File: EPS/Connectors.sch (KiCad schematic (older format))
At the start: 1 part

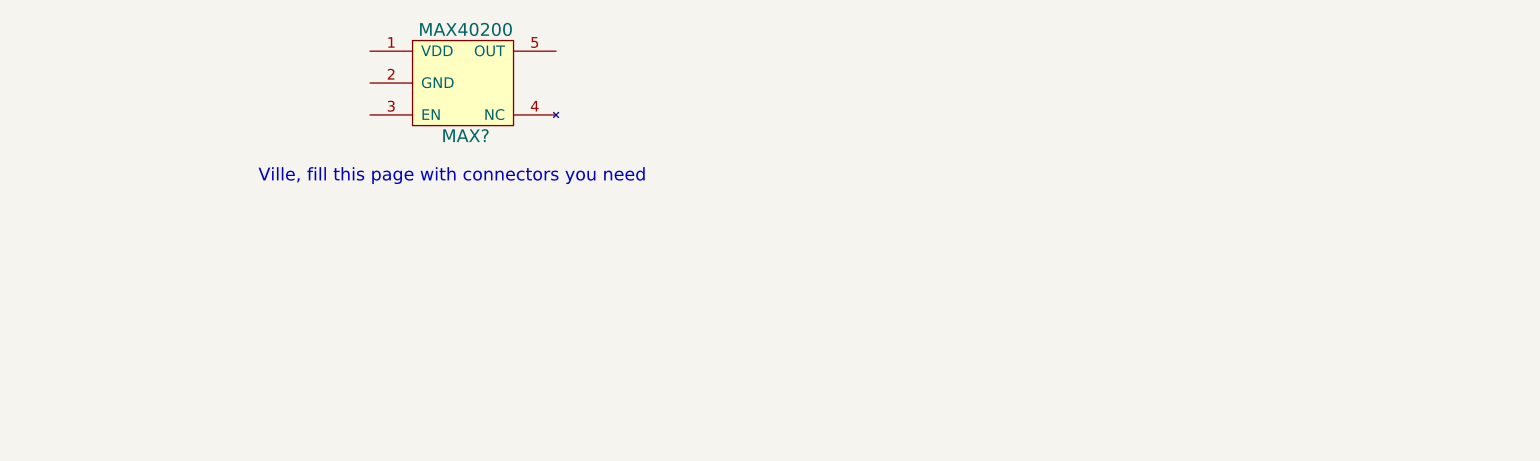
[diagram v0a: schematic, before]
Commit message: Updated schematics
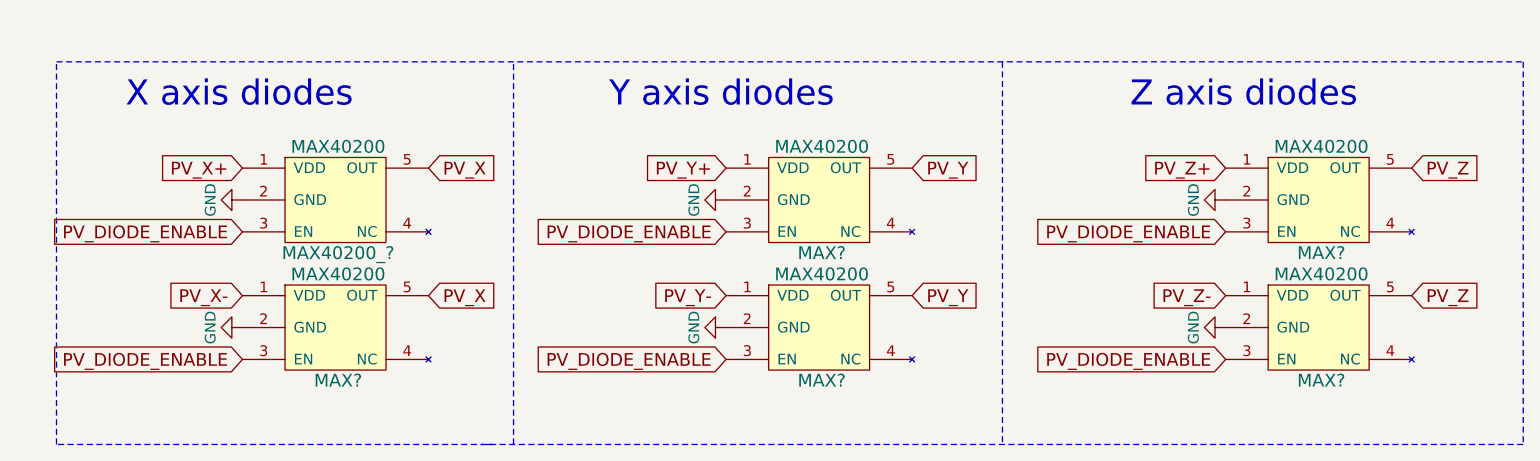
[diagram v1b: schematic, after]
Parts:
- added MAX40200_?, MAX? (x4): MAX40200, symbol MAX40200
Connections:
- net PV_X-: now reaches MAX?.1 (VDD)
- net GND: now reaches MAX?.2 (GND)
- net GND: now also MAX40200_?.2 (GND), MAX?.2 (GND), MAX?.2 (GND), MAX?.2 (GND), MAX?.2 (GND)
- net PV_DIODE_ENABLE: now reaches MAX?.3 (EN)
- net PV_DIODE_ENABLE: now also MAX40200_?.3 (EN), MAX?.3 (EN), MAX?.3 (EN), MAX?.3 (EN), MAX?.3 (EN)
- net PV_X: now reaches MAX?.5 (OUT)
- net PV_X: now also MAX40200_?.5 (OUT)
- new net PV_X+: MAX40200_?.1 (VDD)
- new net PV_Y: MAX?.5 (OUT), MAX?.5 (OUT)
- new net PV_Y+: MAX?.1 (VDD)
- new net PV_Y-: MAX?.1 (VDD)
- new net PV_Z: MAX?.5 (OUT), MAX?.5 (OUT)
- new net PV_Z+: MAX?.1 (VDD)
- new net PV_Z-: MAX?.1 (VDD)
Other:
- note added: "X axis diodes"
- note added: "Y axis diodes"
- note added: "Z axis diodes"
- note removed: "Ville, fill this page with connectors you need\n"
- moved on the sheet: MAX?
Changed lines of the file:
@@
 LIBS:max40200
 LIBS:tps7a7002
+LIBS:max5395
 LIBS:EPS-cache
 EELAYER 25 0
@@
 L MAX40200 MAX?
 U 1 1 5A8C9975
-P 5525 2725
-F 0 "MAX?" H 5525 2450 60  0000 C CNN
-F 1 "MAX40200" H 5525 2950 60  0000 C CNN
-F 2 "" H 5475 2725 60  0001 C CNN
-F 3 "" H 5475 2725 60  0001 C CNN
-	1    5525 2725
-	1    0    0    -1
-$EndComp
-Text Notes 4550 3225 0    60   ~ 0
-Ville, fill this page with connectors you need\n
+P 4925 3875
+F 0 "MAX?" H 4925 3600 60  0000 C CNN
+F 1 "MAX40200" H 4925 4100 60  0000 C CNN
+F 2 "" H 4875 3875 60  0001 C CNN
+F 3 "" H 4875 3875 60  0001 C CNN
+	1    4925 3875
+	1    0    0    -1
+$EndComp
+$Comp
+L MAX40200 MAX40200_?
+U 1 1 5A8B6733
+P 4925 3275
+F 0 "MAX40200_?" H 4925 3000 60  0000 C CNN
+F 1 "MAX40200" H 4925 3500 60  0000 C CNN
+F 2 "" H 4875 3275 60  0001 C CNN
+F 3 "" H 4875 3275 60  0001 C CNN
+	1    4925 3275
+	1    0    0    -1
+$EndComp
+Wire Notes Line
+	3600 2650 10500 2650
+Wire Notes Line
+	10500 2650 10500 4450
+Wire Notes Line
+	10500 4450 3600 4450
+Wire Notes Line
+	3600 4450 3600 2650
+Wire Notes Line
+	5650 4450 5600 4450
+Wire Notes Line
+	8050 2650 8050 4450
+$Comp
+L MAX40200 MAX?
+U 1 1 5A8B6858
+P 7200 3875
+F 0 "MAX?" H 7200 3600 60  0000 C CNN
+F 1 "MAX40200" H 7200 4100 60  0000 C CNN
+F 2 "" H 7150 3875 60  0001 C CNN
+F 3 "" H 7150 3875 60  0001 C CNN
+	1    7200 3875
+	1    0    0    -1
+$EndComp
+$Comp
+L MAX40200 MAX?
+U 1 1 5A8B685E
+P 7200 3275
+F 0 "MAX?" H 7200 3000 60  0000 C CNN
+F 1 "MAX40200" H 7200 3500 60  0000 C CNN
+F 2 "" H 7150 3275 60  0001 C CNN
+F 3 "" H 7150 3275 60  0001 C CNN
+	1    7200 3275
+	1    0    0    -1
+$EndComp
+$Comp
+L MAX40200 MAX?
+U 1 1 5A8B6906
+P 9550 3875
+F 0 "MAX?" H 9550 3600 60  0000 C CNN
+F 1 "MAX40200" H 9550 4100 60  0000 C CNN
+F 2 "" H 9500 3875 60  0001 C CNN
+F 3 "" H 9500 3875 60  0001 C CNN
+	1    9550 3875
+	1    0    0    -1
+$EndComp
+$Comp
+L MAX40200 MAX?
+U 1 1 5A8B690C
+P 9550 3275
+F 0 "MAX?" H 9550 3000 60  0000 C CNN
+F 1 "MAX40200" H 9550 3500 60  0000 C CNN
+F 2 "" H 9500 3275 60  0001 C CNN
+F 3 "" H 9500 3275 60  0001 C CNN
+	1    9550 3275
+	1    0    0    -1
+$EndComp
+Text GLabel 4475 3150 0    60   Input ~ 0
+PV_X+
+Text GLabel 4475 3750 0    60   Input ~ 0
+PV_X-
+Text GLabel 6750 3150 0    60   Input ~ 0
+PV_Y+
+Text GLabel 6750 3750 0    60   Input ~ 0
+PV_Y-
+Text GLabel 9100 3150 0    60   Input ~ 0
+PV_Z+
+Text GLabel 9100 3750 0    60   Input ~ 0
+PV_Z-
+Text GLabel 5350 3150 2    60   Input ~ 0
+PV_X
+Text GLabel 5350 3750 2    60   Input ~ 0
+PV_X
+Text GLabel 7625 3150 2    60   Input ~ 0
+PV_Y
+Text GLabel 7625 3750 2    60   Input ~ 0
+PV_Y
+Text GLabel 9975 3150 2    60   Input ~ 0
+PV_Z
+Text GLabel 9975 3750 2    60   Input ~ 0
+PV_Z
+$Comp
+L GND #PWR?
+U 1 1 5A8B7527
+P 4475 3300
+F 0 "#PWR?" H 4475 3050 50  0001 C CNN
+F 1 "GND" H 4475 3150 50  0000 C CNN
+F 2 "" H 4475 3300 50  0001 C CNN
+F 3 "" H 4475 3300 50  0001 C CNN
+	1    4475 3300
+	0    1    1    0
+$EndComp
+$Comp
+L GND #PWR?
+U 1 1 5A8B755E
+P 4475 3900
+F 0 "#PWR?" H 4475 3650 50  0001 C CNN
+F 1 "GND" H 4475 3750 50  0000 C CNN
+F 2 "" H 4475 3900 50  0001 C CNN
+F 3 "" H 4475 3900 50  0001 C CNN
+	1    4475 3900
+	0    1    1    0
+$EndComp
+$Comp
+L GND #PWR?
+U 1 1 5A8B757B
+P 6750 3300
+F 0 "#PWR?" H 6750 3050 50  0001 C CNN
+F 1 "GND" H 6750 3150 50  0000 C CNN
+F 2 "" H 6750 3300 50  0001 C CNN
+F 3 "" H 6750 3300 50  0001 C CNN
+	1    6750 3300
+	0    1    1    0
+$EndComp
+$Comp
+L GND #PWR?
+U 1 1 5A8B7598
+P 6750 3900
+F 0 "#PWR?" H 6750 3650 50  0001 C CNN
+F 1 "GND" H 6750 3750 50  0000 C CNN
+F 2 "" H 6750 3900 50  0001 C CNN
+F 3 "" H 6750 3900 50  0001 C CNN
+	1    6750 3900
+	0    1    1    0
+$EndComp
+$Comp
+L GND #PWR?
+U 1 1 5A8B75B5
+P 9100 3300
+F 0 "#PWR?" H 9100 3050 50  0001 C CNN
+F 1 "GND" H 9100 3150 50  0000 C CNN
+F 2 "" H 9100 3300 50  0001 C CNN
+F 3 "" H 9100 3300 50  0001 C CNN
+	1    9100 3300
+	0    1    1    0
+$EndComp
+$Comp
+L GND #PWR?
+U 1 1 5A8B75D2
+P 9100 3900
+F 0 "#PWR?" H 9100 3650 50  0001 C CNN
+F 1 "GND" H 9100 3750 50  0000 C CNN
+F 2 "" H 9100 3900 50  0001 C CNN
+F 3 "" H 9100 3900 50  0001 C CNN
+	1    9100 3900
+	0    1    1    0
+$EndComp
+Text GLabel 4475 3450 0    60   Input ~ 0
+PV_DIODE_ENABLE
+Text GLabel 4475 4050 0    60   Input ~ 0
+PV_DIODE_ENABLE
+Text GLabel 6750 4050 0    60   Input ~ 0
+PV_DIODE_ENABLE
+Text GLabel 6750 3450 0    60   Input ~ 0
+PV_DIODE_ENABLE
+Text GLabel 9100 3450 0    60   Input ~ 0
+PV_DIODE_ENABLE
+Text GLabel 9100 4050 0    60   Input ~ 0
+PV_DIODE_ENABLE
+Text Notes 3925 2875 0    118  ~ 0
+X axis diodes
+Text Notes 6200 2875 0    118  ~ 0
+Y axis diodes
+Text Notes 8650 2875 0    118  ~ 0
+Z axis diodes
+Wire Notes Line
+	5750 4450 5750 2650
 $EndSCHEMATC
